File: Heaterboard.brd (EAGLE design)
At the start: 132.1 x 36.5 mm, 14 parts, among them IC1 EK-TM4C123GXLP, J1 POWER_JACK, U1 CSD18504KCS, U2 LM35DT

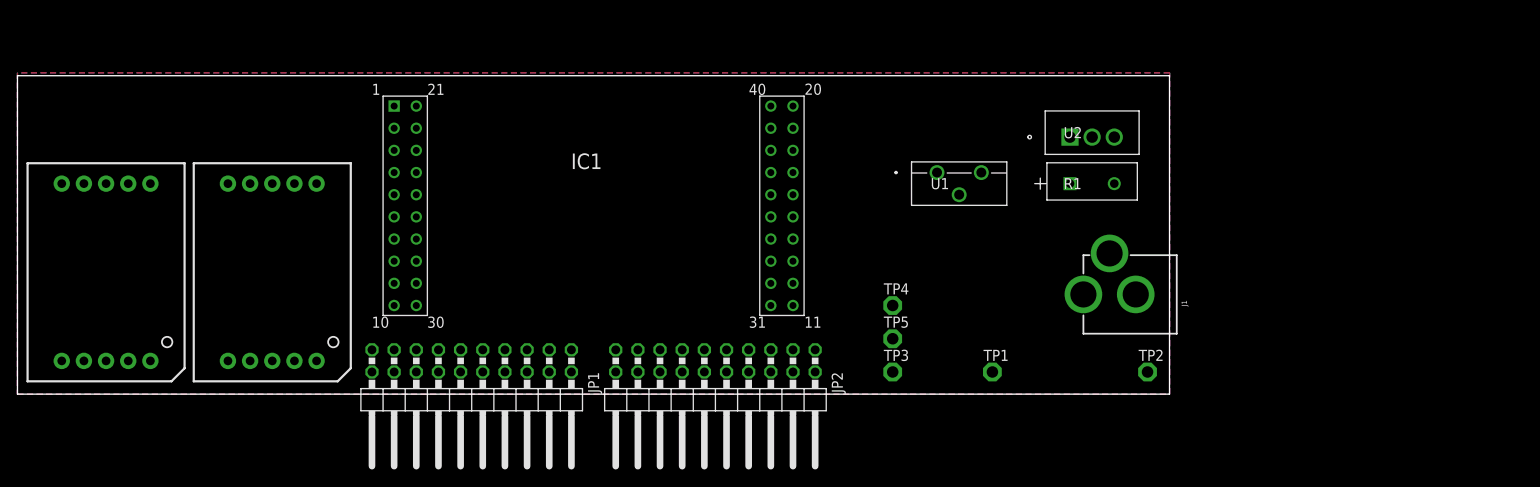
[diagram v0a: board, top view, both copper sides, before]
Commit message: checkpoint for schematic capture
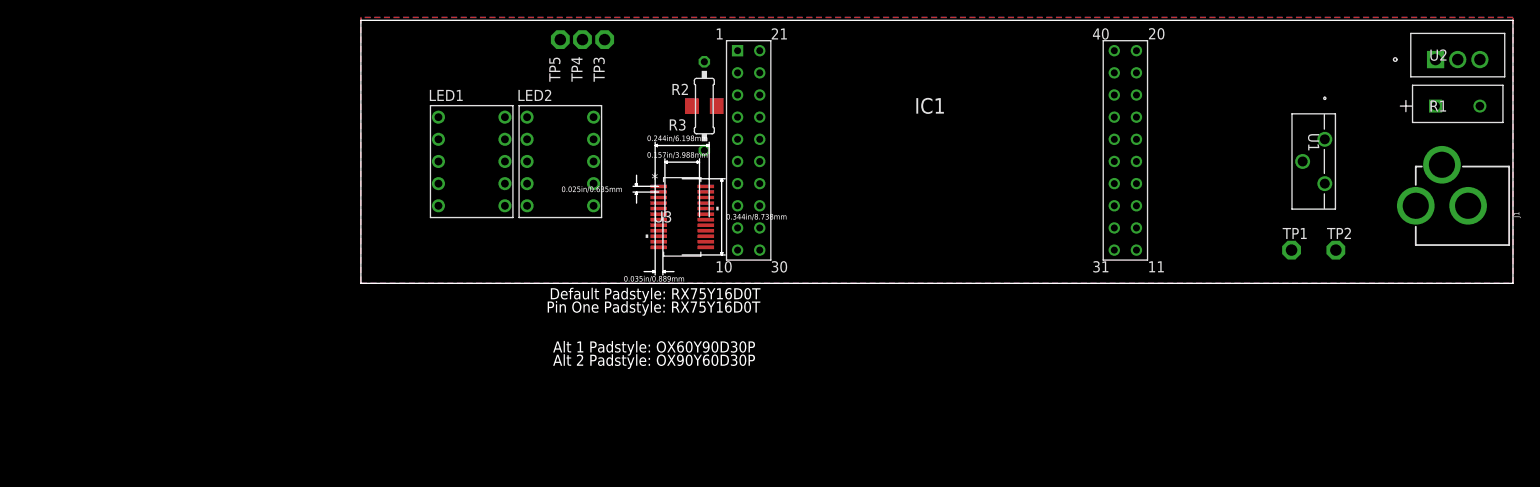
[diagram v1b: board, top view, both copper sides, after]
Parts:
- removed JP1, JP2: (no value), pinhead:2X10/90
- removed U$1, U$2: YSD-160AB3C-8, SparkFun-LED:7-SEGMENT-1"PTH
- added LED1, LED2: LA-401AD, led-7-segment:LA-401
- added R2: (no value), resistor:R1206
- added R3: (no value), resistor:0207/10
- added U3: TLC5926IDBQRDBQ24-M, partlibrary:DBQ24-M
- moved TP5 51.3 mm to (22.9, 34.3)
- moved TP3 50.4 mm to (27.9, 34.3)
- moved TP4 46.8 mm to (25.4, 34.3)
- moved R1 42.8 mm to (128.3, 26.7)
- moved U2 42.8 mm to (128.3, 33.0)
- moved IC1 39.9 mm to (66.0, 20.3)
- moved J1 39.4 mm to (134.6, 15.2)
- moved TP1 37.0 mm to (106.7, 10.2)
- moved U1 36.9 mm to (108.0, 17.8), turned to 270 degrees
- moved TP2 25.7 mm to (111.8, 10.2)
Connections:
- removed net N$2: IC1.2, JP1.3
- removed net N$21: IC1.36, JP2.9
- removed net N$22: IC1.35, JP2.11
- removed net N$23: IC1.34, JP2.13
- removed net N$24: IC1.33, JP2.15
- removed net N$25: IC1.32, JP2.17
- removed net N$26: IC1.31, JP2.19
- removed net N$27: IC1.19, JP2.4
- removed net N$28: IC1.18, JP2.6
- removed net N$29: IC1.17, JP2.8
- removed net N$3: IC1.3, JP1.5
- removed net N$30: IC1.16, JP2.10
- removed net N$31: IC1.15, JP2.12
- removed net N$32: IC1.14, JP2.14
- removed net N$33: IC1.13, JP2.16
- removed net N$34: IC1.12, JP2.18
- removed net N$35: IC1.11, JP2.20
- removed net N$4: IC1.4, JP1.7
- new net CLK: IC1.23, U3.3
- new net FSS: IC1.24
- new net LE: U3.4
- new net N$40: R2.1, R3.1, U3.23
- new net OE: U3.21
- new net SDI: IC1.26, U3.2
- new net SDO: IC1.25, U3.22
- net +3V3: now also LED1.1, LED1.6, LED2.1, LED2.6; no longer JP1.1
- net +5V: now also U3.24; no longer JP1.2
- net GND: now also R2.2, R3.2, U3.1; no longer JP1.4, JP2.2
- net N$10: now also LED1.2, U3.10; no longer IC1.10, JP1.19
- net N$11: now also LED1.3, U3.11; no longer IC1.23, JP1.6
- net N$12: now also LED1.7, U3.12; no longer IC1.24, JP1.8
- net N$13: now also LED2.7, U3.13; no longer IC1.25, JP1.10
- net N$14: now also LED2.3, U3.14; no longer IC1.26, JP1.12
- net N$15: now also LED2.2, U3.15; no longer IC1.28, JP1.16
- net N$16: now also LED2.4, U3.16; no longer IC1.30, JP1.20
- net N$17: now also LED2.5, U3.17; no longer IC1.40, JP2.1
- net N$18: now also LED2.8, U3.18; no longer IC1.39, JP2.3
- net N$19: now also LED2.9, U3.19; no longer IC1.38, JP2.5
- net N$20: now also LED2.10, U3.20; no longer IC1.37, JP2.7
- net N$5: now also LED1.10, U3.5; no longer IC1.5, JP1.9
- net N$6: now also LED1.9, U3.6; no longer IC1.6, JP1.11
- net N$7: now also LED1.8, U3.7; no longer IC1.7, JP1.13
- net N$8: now also LED1.5, U3.8; no longer IC1.8, JP1.15
- net N$9: now also LED1.4, U3.9; no longer IC1.9, JP1.17
- net PWR_ON: no longer JP1.14
- net T-SENSE: no longer JP1.18
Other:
- board size 132.1 x 36.5 mm -> 132.1 x 30.1 mm
